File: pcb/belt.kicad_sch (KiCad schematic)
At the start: 0 parts

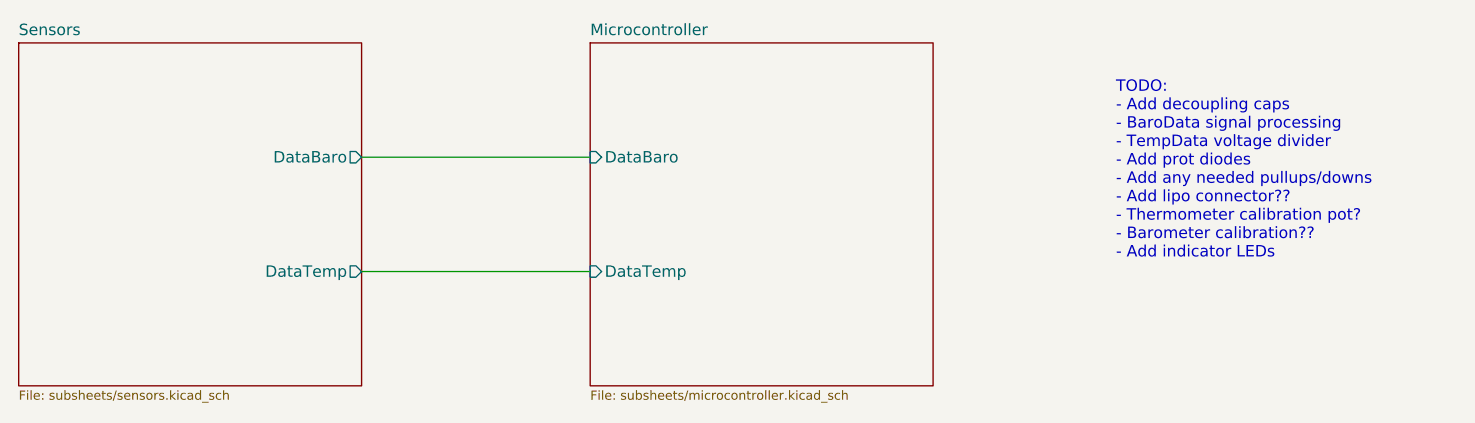
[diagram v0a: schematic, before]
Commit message: fixed everything (ERC is no longer mad)
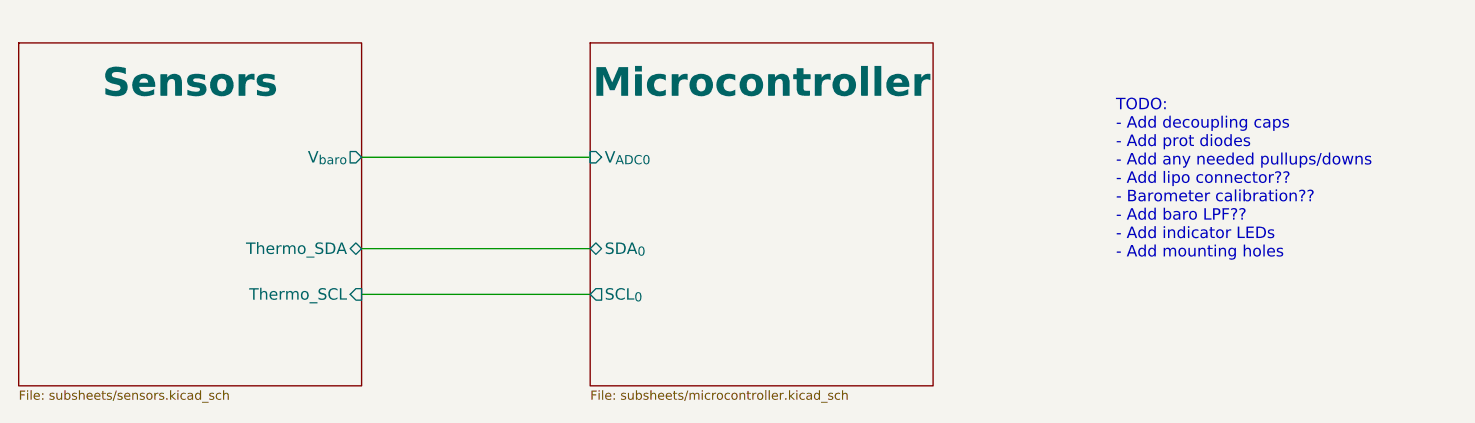
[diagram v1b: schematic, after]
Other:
- sheet Microcontroller ports: added SCL_{0}, SDA_{0}, V_{ADC0}; removed DataBaro, DataTemp
- sheet Sensors ports: added Thermo_SCL, Thermo_SDA, V_{baro}; removed DataBaro, DataTemp
- note added: "TODO: - Add decoupling caps - Add prot diodes - Add any needed pullups/downs - Add lipo connector?? - Barometer calibration?? - Add baro LPF?? - Add indicator LEDs - Add mounting holes"
- note removed: "TODO: - Add decoupling caps - BaroData signal processing - TempData voltage divider - Add prot diodes - Add any needed pullups/downs - Add lipo connector?? - Thermometer calibration pot? - Barometer calibration?? - Add indicator LEDs"
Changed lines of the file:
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@@
   (title_block
     (title "Basic Electronics Learning Toolkit")
-    (date "2023-12-27")
-    (rev "0.1")
+    (date "2023-12-31")
+    (rev "0.2")
     (company "Rice Eclipse")
+    (comment 1 "Adam Sher")
   )
-  (wire (pts (xy 101.6 88.9) (xy 127 88.9))
+  (wire (pts (xy 101.6 91.44) (xy 127 91.44))
+    (stroke (width 0) (type default))
+  )
+  (wire (pts (xy 101.6 86.36) (xy 127 86.36))
     (stroke (width 0) (type default))
   )
@@
     (stroke (width 0) (type default))
   )
-  (text "TODO: \n- Add decoupling caps\n- BaroData signal processing\n- TempData voltage divider\n- Add prot diodes\n- Add any needed pullups/downs\n- Add lipo connector??\n- Thermometer calibration pot?\n- Barometer calibration??\n- Add indicator LEDs"
+  (text "TODO: \n- Add decoupling caps\n- Add prot diodes\n- Add any needed pullups/downs\n- Add lipo connector??\n- Barometer calibration??\n- Add baro LPF??\n- Add indicator LEDs\n- Add mounting holes"
     (at 185.42 87.63 0)
     (effects (font (size 1.27 1.27)) (justify left bottom))
   )
-  (sheet (at 127 63.5) (size 38.1 38.1) (fields_autoplaced)
+  (sheet (at 127 63.5) (size 38.1 38.1)
     (stroke (width 0.1524) (type solid))
     (fill (color 0 0 0 0.0000))
-    (property "Sheetname" "Microcontroller" (at 127 62.7884 0)
-      (effects (font (size 1.27 1.27)) (justify left bottom))
+    (property "Sheetname" "Microcontroller" (at 146.05 66.04 0) (do_not_autoplace)
+      (effects (font (size 3.175 3.175) bold) (justify top))
     )
     (property "Sheetfile" "subsheets/microcontroller.kicad_sch" (at 127 102.083 0)
       (effects (font (size 1.016 1.016)) (justify left top))
     )
-    (pin "DataTemp" input (at 127 88.9 180)
+    (pin "V_{ADC0}" input (at 127 76.2 180)
       (effects (font (size 1.27 1.27)) (justify left))
     )
-    (pin "DataBaro" input (at 127 76.2 180)
+    (pin "SDA_{0}" bidirectional (at 127 86.36 180)
+      (effects (font (size 1.27 1.27)) (justify left))
+    )
+    (pin "SCL_{0}" output (at 127 91.44 180)
       (effects (font (size 1.27 1.27)) (justify left))
     )
@@
     )
   )
-  (sheet (at 63.5 63.5) (size 38.1 38.1) (fields_autoplaced)
+  (sheet (at 63.5 63.5) (size 38.1 38.1)
     (stroke (width 0.1524) (type solid))
     (fill (color 0 0 0 0.0000))
-    (property "Sheetname" "Sensors" (at 63.5 62.7884 0)
-      (effects (font (size 1.27 1.27)) (justify left bottom))
+    (property "Sheetname" "Sensors" (at 82.55 66.04 0) (do_not_autoplace)
+      (effects (font (size 3.175 3.175) bold) (justify top))
     )
     (property "Sheetfile" "subsheets/sensors.kicad_sch" (at 63.5 102.083 0)
       (effects (font (size 1.016 1.016)) (justify left top))
     )
-    (pin "DataBaro" output (at 101.6 76.2 0)
+    (pin "V_{baro}" output (at 101.6 76.2 0)
       (effects (font (size 1.27 1.27)) (justify right))
     )
-    (pin "DataTemp" output (at 101.6 88.9 0)
+    (pin "Thermo_SDA" bidirectional (at 101.6 86.36 0)
       (effects (font (size 1.27 1.27)) (justify right))
     )
+    (pin "Thermo_SCL" input (at 101.6 91.44 0)
+      (effects (font (size 1.27 1.27)) (justify right))
+    )
